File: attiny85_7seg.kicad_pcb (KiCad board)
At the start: 2 copper layers, 55 x 55 mm, 16 parts, among them J1 Conn_01x06_Pin, J2 Conn_01x03_Pin, U1 ATtiny85-20P, U2 CC56-12SURKWA, U3 74HC595, U4 74HC595

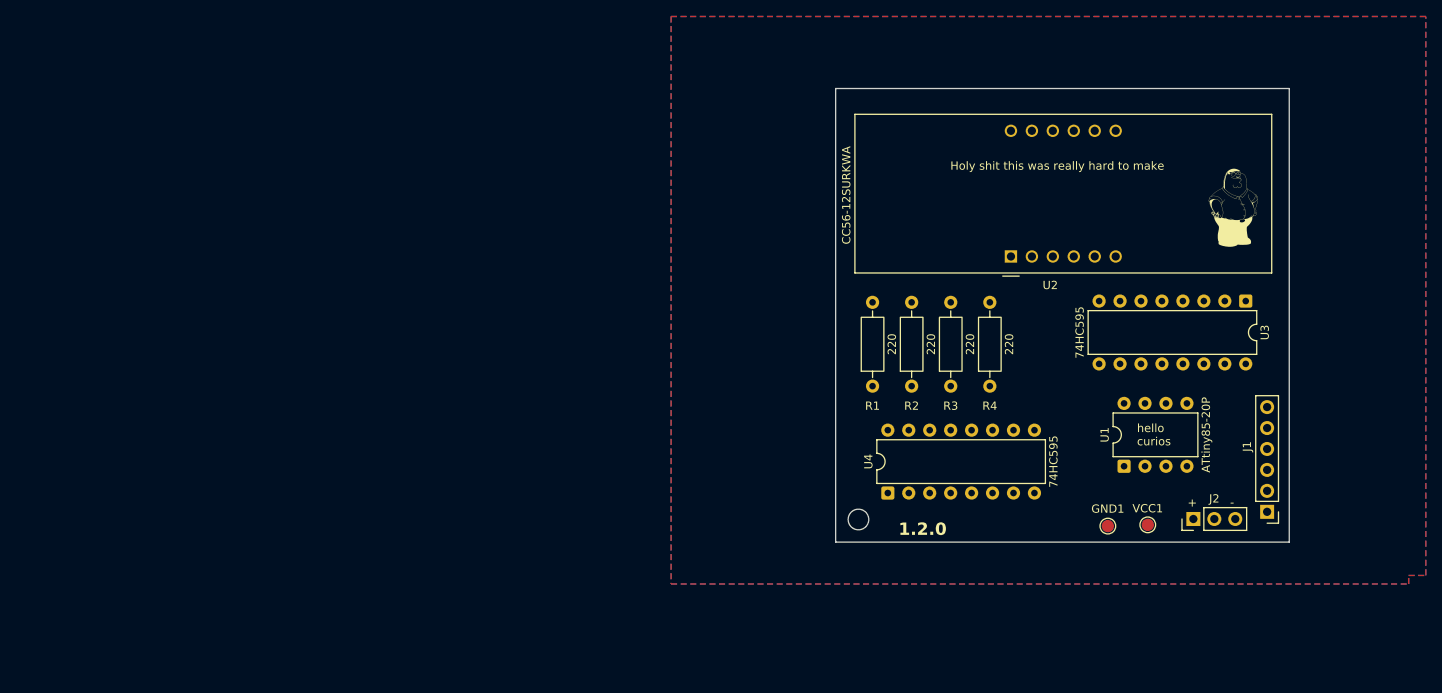
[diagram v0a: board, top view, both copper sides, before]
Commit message: 0.0.3
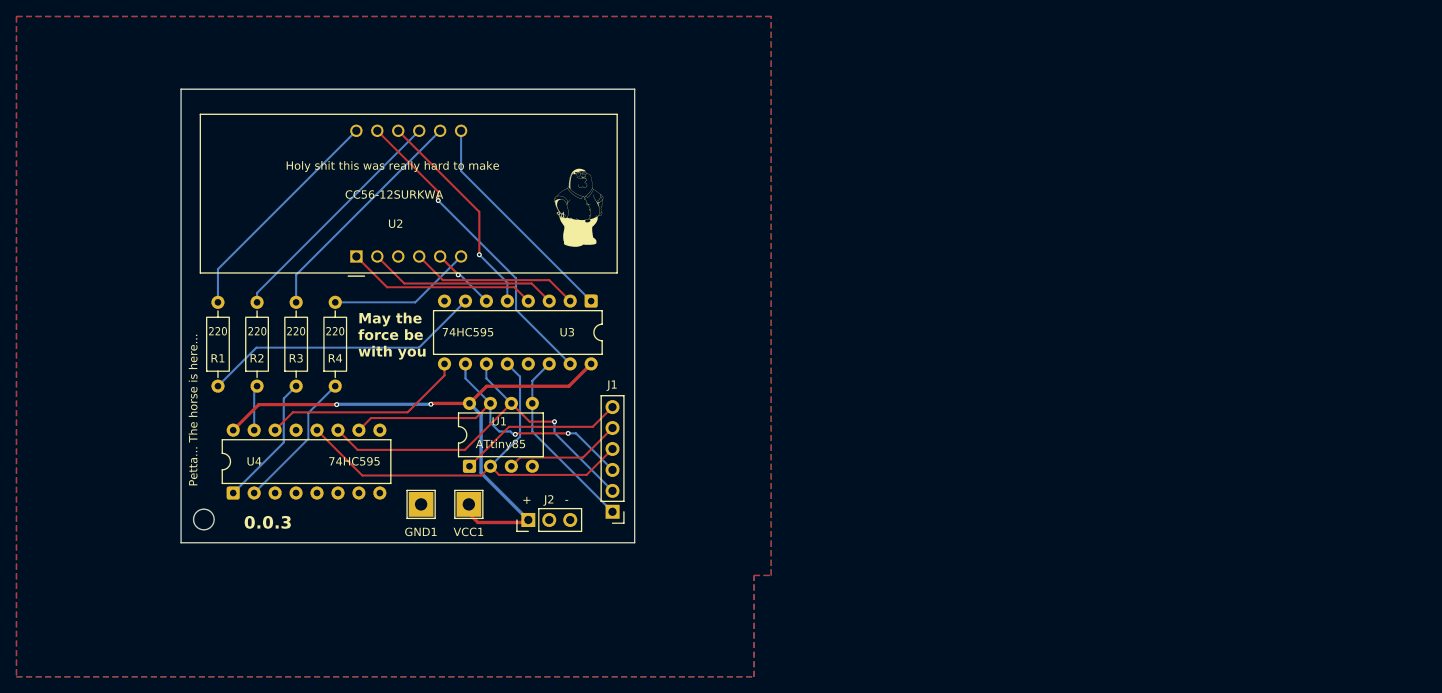
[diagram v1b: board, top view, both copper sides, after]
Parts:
- added LOGO1: LOGO, SilkScreen:thehorseishere, B.Cu at (144.9, 92.7)
- GND1, VCC1: footprint TestPoint:TestPoint_Pad_D1.5mm -> TestPoint:TestPoint_THTPad_3.0x3.0mm_Drill1.5mm
- U1: value ATtiny85-20P -> ATtiny85
- moved GND1 83.3 mm to (133.6, 103.6)
- moved VCC1 82.4 mm to (139.4, 103.6)
- moved IMG2 80.8 mm to (109.3, 64.3)
- moved J2 80.6 mm to (146.6, 105.5)
- moved IMG1 79.4 mm to (152.7, 67.7)
- moved J1 79.4 mm to (156.8, 104.5)
- moved R1 79.4 mm to (108.9, 89.3)
- moved R2 79.4 mm to (113.7, 89.3)
- moved R4 79.4 mm to (123.2, 89.3)
- moved U1 79.4 mm to (139.4, 99.0)
- moved U2 79.4 mm to (125.7, 73.6)
- moved U3 79.4 mm to (154.2, 79.0)
- moved HOLE1 79.4 mm to (107.2, 105.5)
- moved R3 79.4 mm to (118.4, 89.3)
- moved U4 79.4 mm to (110.8, 102.3)
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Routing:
- net VCC: track 0.00 -> 71.6 mm, vias 0 -> 2
- net /PB3: track 0.00 -> 54.8 mm
- net /PB1: track 0.00 -> 47.8 mm, vias 0 -> 1
- net /PB2: track 0.00 -> 42.9 mm, vias 0 -> 2
- net Net-(U2-a): track 0.00 -> 38.0 mm, vias 0 -> 1
- net Net-(U3-QH): track 0.00 -> 34.3 mm
- net Net-(U2-CC2): track 0.00 -> 28.9 mm
- net Net-(U2-CC3): track 0.00 -> 28.0 mm
- net Net-(U2-CC1): track 0.00 -> 27.8 mm
- net Net-(U2-b): track 0.00 -> 27.2 mm
- net Net-(U2-f): track 0.00 -> 26.1 mm, vias 0 -> 1
- net Net-(U3-QH'): track 0.00 -> 24.7 mm
- net Net-(U2-d): track 0.00 -> 23.1 mm
- net Net-(U2-e): track 0.00 -> 23.1 mm
- net /PB0: track 0.00 -> 22.8 mm
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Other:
- board text added: "May the force be with you"
- board text added: "Petta... The horse is here..."
- board text added: "With great power comes great responsibility"
- board text removed: "hello curios"

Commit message: 0.0.4
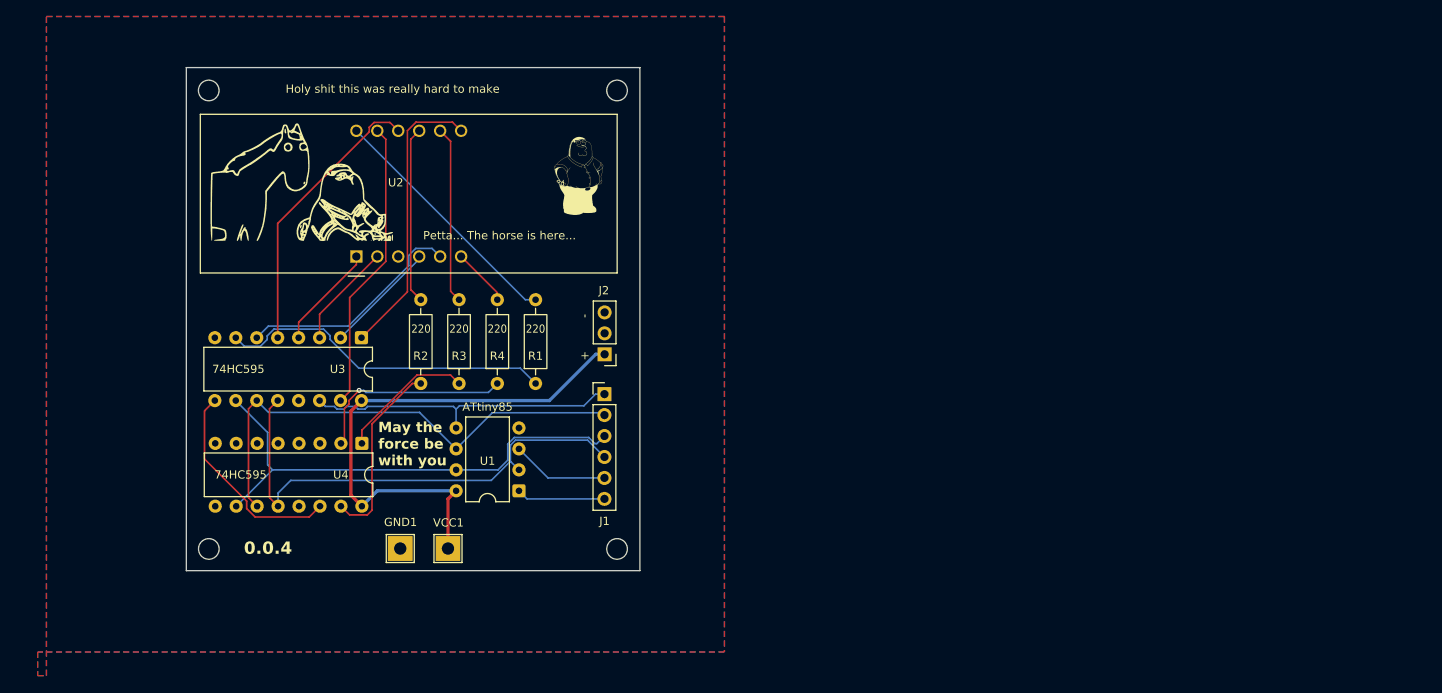
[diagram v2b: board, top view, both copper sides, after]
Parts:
- added HOLE2: MountingHole_2.5mm, MountingHole:MountingHole_2.5mm, F.Cu at (157.3, 109.0)
- added HOLE3: MountingHole_2.5mm, MountingHole:MountingHole_2.5mm, F.Cu at (157.3, 53.5)
- added HOLE4: MountingHole_2.5mm, MountingHole:MountingHole_2.5mm, F.Cu at (107.8, 53.5)
- added IMG5: LOGO, SilkScreen:simbols, B.Cu at (130.0, 91.5)
- LOGO1: moved to F.Cu
- moved LOGO1 41.8 mm to (117.0, 61.6), turned to 0 degrees
- moved R1 38.5 mm to (147.4, 89.0)
- moved U3 28.2 mm to (126.3, 83.4)
- moved J2 22.1 mm to (155.8, 85.4), turned to 180 degrees
- moved R2 19.9 mm to (133.5, 89.0)
- moved R3 19.8 mm to (138.2, 89.0)
- moved R4 19.7 mm to (142.8, 89.0)
- moved U4 16.7 mm to (126.4, 96.2), turned to -90 degrees
- moved J1 14.3 mm to (155.8, 90.3), turned to 0 degrees
- moved IMG3 6.81 mm to (155.6, 67.1)
- moved U1 6.70 mm to (145.4, 102.0), turned to 180 degrees
- moved GND1 5.92 mm to (131.0, 109.0)
- moved VCC1 5.92 mm to (136.8, 109.0)
- moved IMG1 3.86 mm to (152.7, 63.8)
- moved HOLE1 3.62 mm to (107.8, 109.0)
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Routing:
- net Net-(U2-g): track 7.87 -> 27.9 mm, vias 1 -> 0
- net Net-(U4-QA): track 5.48 -> 22.8 mm
- net /PB2: track 42.9 -> 60.2 mm, vias 2 -> 0
- net /PB0: track 22.8 -> 38.5 mm
- net /PB1: track 47.8 -> 60.2 mm, vias 1 -> 0
- net Net-(U2-CC4): track 17.6 -> 7.06 mm
- net Net-(U2-d): track 23.1 -> 12.7 mm
- net Net-(U2-e): track 23.1 -> 12.7 mm
- net /PB5: track 20.3 -> 10.8 mm
- net Net-(U2-f): track 26.1 -> 34.3 mm, vias 1 -> 0
- net Net-(U4-QC): track 17.0 -> 24.6 mm, vias 0 -> 1
- net Net-(U2-b): track 27.2 -> 34.8 mm
- net Net-(U2-CC2): track 28.9 -> 21.4 mm
- net Net-(U2-c): track 20.5 -> 13.8 mm
- net Net-(U3-QH): track 34.3 -> 40.9 mm
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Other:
- board size 55 x 55 mm -> 55 x 61 mm
